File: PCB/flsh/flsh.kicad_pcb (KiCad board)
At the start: 2 copper layers, 40 x 40 mm, 10 parts, among them U1 0.18Ω, U2 0.18Ω, U3 0.18Ω, U4 0.18Ω, U5 0.18Ω

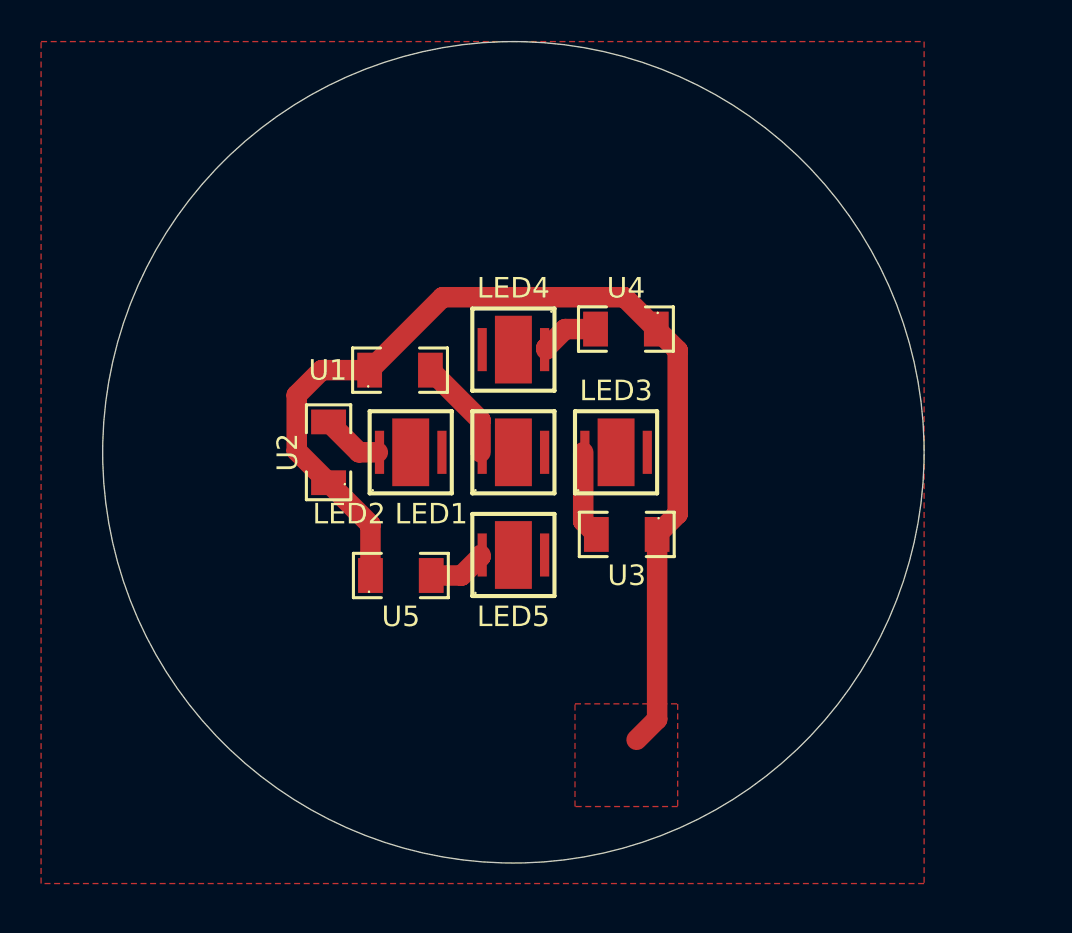
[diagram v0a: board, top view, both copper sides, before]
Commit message: flsh!!
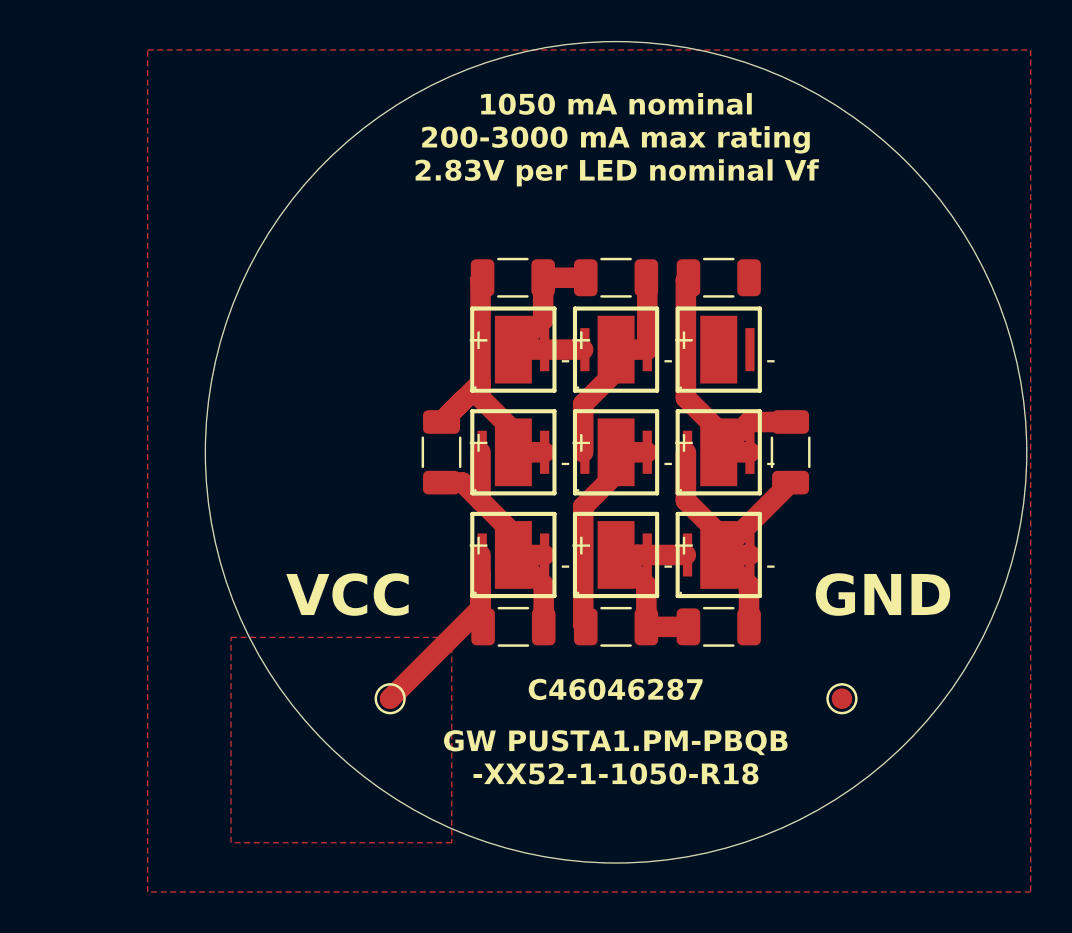
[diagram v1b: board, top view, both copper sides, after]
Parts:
- removed U1, U2, U3, U4, U5: 0.18Ω, easyeda2kicad:R1206
- added C1: C_US, Capacitor_SMD:C_1206_3216Metric, F.Cu at (48.0, 44.5)
- added C2: C_US, Capacitor_SMD:C_1206_3216Metric, F.Cu at (48.0, 27.5)
- added C3: C_US, Capacitor_SMD:C_1206_3216Metric, F.Cu at (58.0, 44.5)
- added C4: C_US, Capacitor_SMD:C_1206_3216Metric, F.Cu at (58.0, 27.5)
- added C5: C_US, Capacitor_SMD:C_1206_3216Metric, F.Cu at (44.5, 36.0)
- added C6: C_US, Capacitor_SMD:C_1206_3216Metric, F.Cu at (53.0, 27.5)
- added C7: C_US, Capacitor_SMD:C_1206_3216Metric, F.Cu at (53.0, 44.5)
- added C8: C_US, Capacitor_SMD:C_1206_3216Metric, F.Cu at (61.5, 36.0)
- added LED6: GW PUSTA1.PM-PBQB-XX52-1-1050-R18, easyeda2kicad:LED-SMD_3P-L3.7-W3.7_GW-PUSTA1.PM-NAPD-XX510-1-1050-R18, F.Cu at (48.0, 41.0)
- added LED7: GW PUSTA1.PM-PBQB-XX52-1-1050-R18, easyeda2kicad:LED-SMD_3P-L3.7-W3.7_GW-PUSTA1.PM-NAPD-XX510-1-1050-R18, F.Cu at (48.0, 36.0)
- added LED8: GW PUSTA1.PM-PBQB-XX52-1-1050-R18, easyeda2kicad:LED-SMD_3P-L3.7-W3.7_GW-PUSTA1.PM-NAPD-XX510-1-1050-R18, F.Cu at (58.0, 36.0)
- added LED9: GW PUSTA1.PM-PBQB-XX52-1-1050-R18, easyeda2kicad:LED-SMD_3P-L3.7-W3.7_GW-PUSTA1.PM-NAPD-XX510-1-1050-R18, F.Cu at (58.0, 31.0)
- added TP1: TestPoint, TestPoint:TestPoint_Pad_D1.0mm, F.Cu at (42.0, 48.0)
- added TP2: TestPoint, TestPoint:TestPoint_Pad_D1.0mm, F.Cu at (64.0, 48.0)
- moved LED2 11.2 mm to (53.0, 31.0)
- moved LED4 11.2 mm to (53.0, 41.0), turned to 0 degrees
- moved LED5 10.0 mm to (58.0, 41.0)
- moved LED1 5.00 mm to (48.0, 31.0)
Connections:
- LED1 pad 2: GND -> Net-(LED2-A)
- LED1 pad 3: GND -> Net-(LED2-A)
- LED2 pad 2: GND -> Net-(LED3-A)
- LED2 pad 3: GND -> Net-(LED3-A)
- LED3 pad 2: GND -> Net-(LED4-A)
- LED3 pad 3: GND -> Net-(LED4-A)
- LED4 pad 2: GND -> Net-(LED5-A)
- LED4 pad 3: GND -> Net-(LED5-A)
- LED5 pad 2: GND -> Net-(LED8-A)
- LED5 pad 3: GND -> Net-(LED8-A)
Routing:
- net LED_VCC: track 51.7 -> 11.4 mm
- net Net-(LED8-A): track 0.00 -> 16.3 mm
- net Net-(LED9-A): track 0.00 -> 14.8 mm
- net Net-(LED7-A): track 0.00 -> 13.6 mm
- net Net-(LED1-A): track 5.01 -> 15.1 mm
- net Net-(LED4-A): track 2.86 -> 10.7 mm
- net Net-(LED5-A): track 2.86 -> 10.1 mm
- net Net-(LED2-A): track 3.01 -> 9.58 mm
- net Net-(LED3-A): track 4.81 -> 10.7 mm
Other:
- board text added: "1050 mA nominal 200-3000 mA max rating 2.83V per LED nominal Vf"
- board text added: "C46046287"
- board text added: "GND"
- board text added: "GW PUSTA1.PM-PBQB -XX52-1-1050-R18"
- board text added: "VCC"
